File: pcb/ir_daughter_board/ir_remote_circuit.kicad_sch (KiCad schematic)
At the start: 12 parts, among them J2 Conn_01x12, J3 Conn_01x12, SW1 BOOT, SW2 RESET, U2 ESP32-WROOM-32E_(16MB)

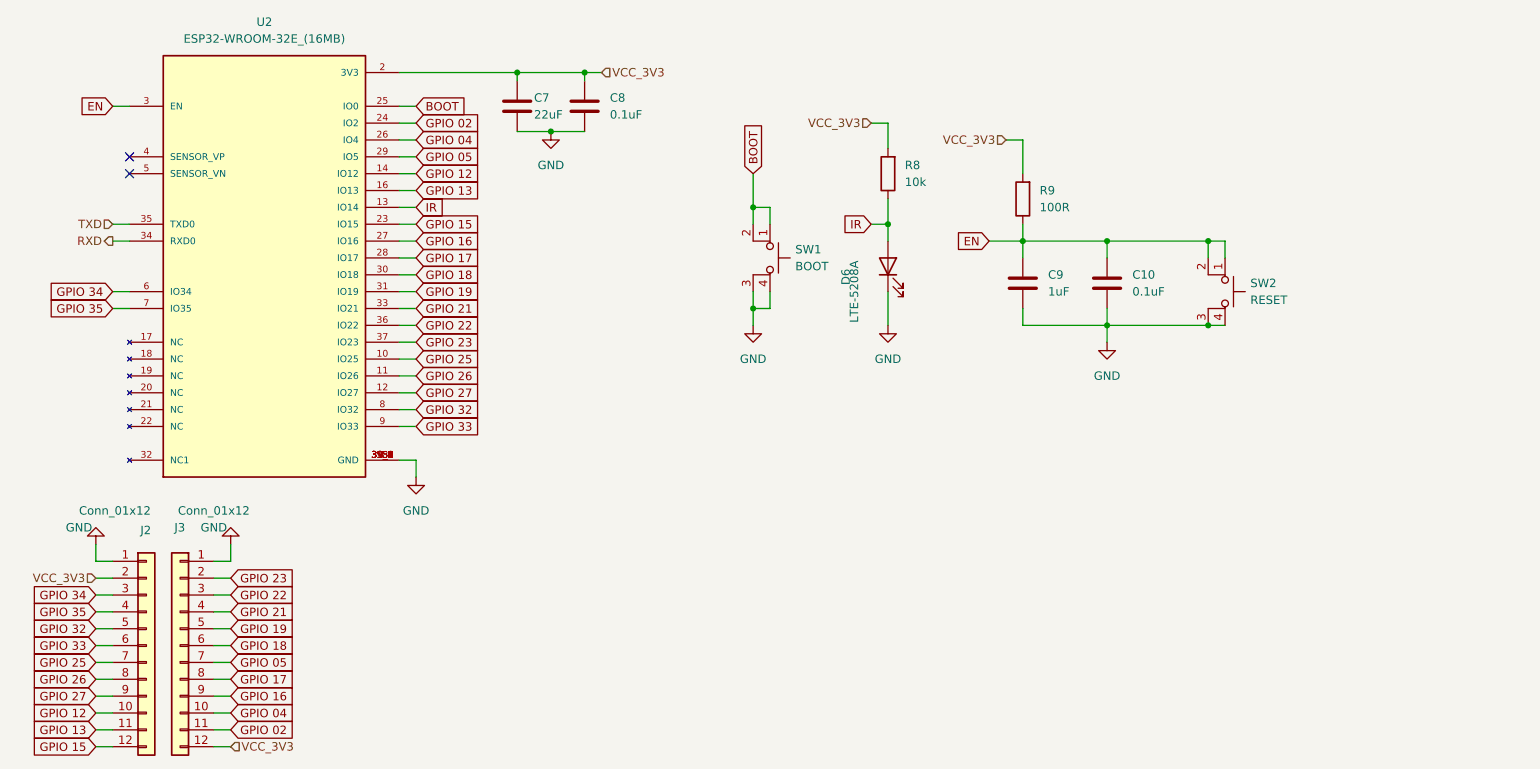
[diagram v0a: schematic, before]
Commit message: minor editorial changes
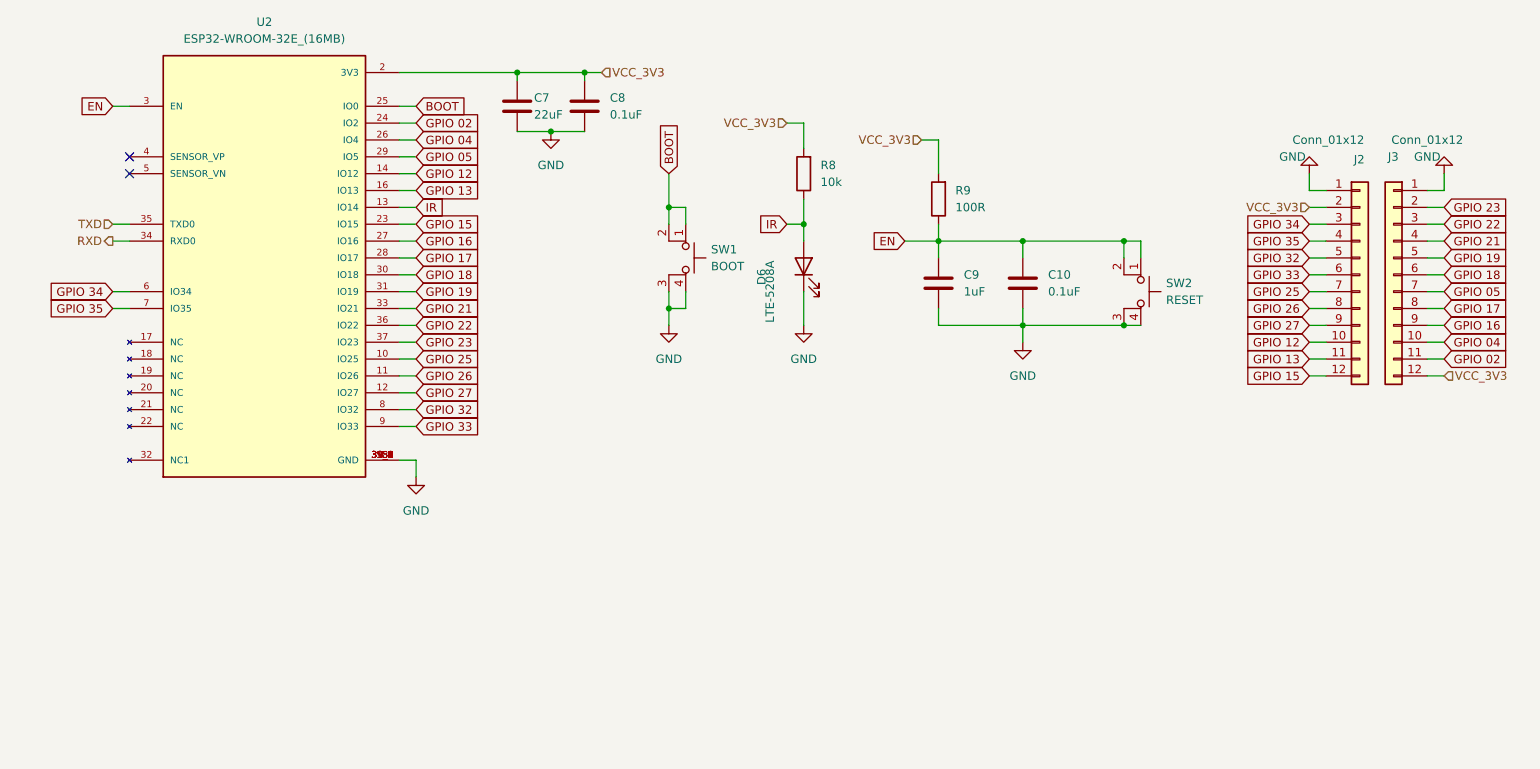
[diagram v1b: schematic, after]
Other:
- moved on the sheet: C10, C9, D6, J2, J3, R8, R9, SW1, SW2
